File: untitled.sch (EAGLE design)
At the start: 1 part

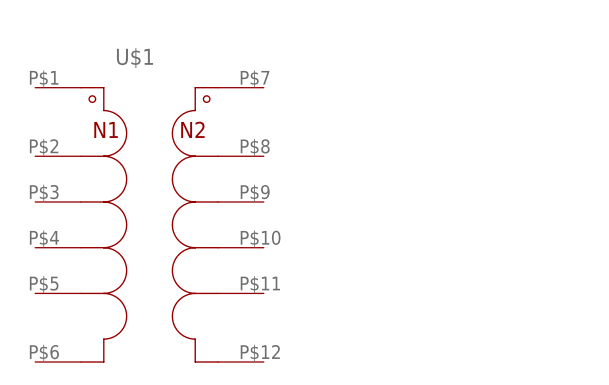
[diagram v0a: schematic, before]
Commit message: add
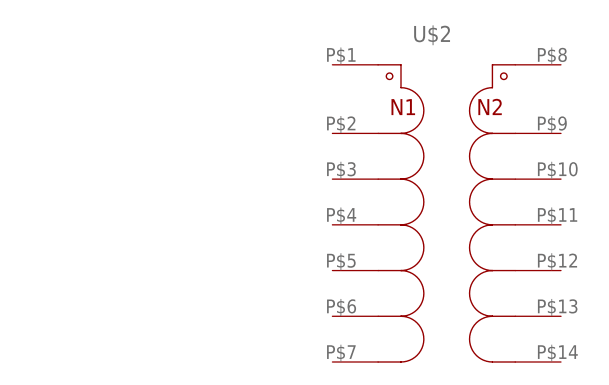
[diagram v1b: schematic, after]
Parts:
- removed U$1: TRANSFORMER-EE40, untitled:TRANSFORMER-EE40
- added U$2: TRANSFORMER-EE40-DOWN, untitled:TRANSFORMER-EE40-DOWN
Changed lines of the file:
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@@
 </classes>
 <parts>
-<part name="U$1" library="untitled" deviceset="TRANSFORMER-EE40" device=""/>
+<part name="U$2" library="untitled" deviceset="TRANSFORMER-EE40-DOWN" device=""/>
 </parts>
 <sheets>
@@
 </plain>
 <instances>
-<instance part="U$1" gate="G$1" x="35.56" y="33.02" smashed="yes">
-<attribute name="NAME" x="31.75" y="45.72" size="1.778" layer="95"/>
+<instance part="U$2" gate="G$1" x="68.58" y="30.48" smashed="yes">
+<attribute name="NAME" x="64.77" y="48.26" size="1.778" layer="95"/>
 </instance>
 </instances>
